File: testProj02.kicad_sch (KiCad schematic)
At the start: 25 parts, among them U1 24LC1025, U2 DS1337S_, U3 24LC1025, U4 ATMEGA328P-AU, Y1 32.768 KHZ, Y2 16 Mhz

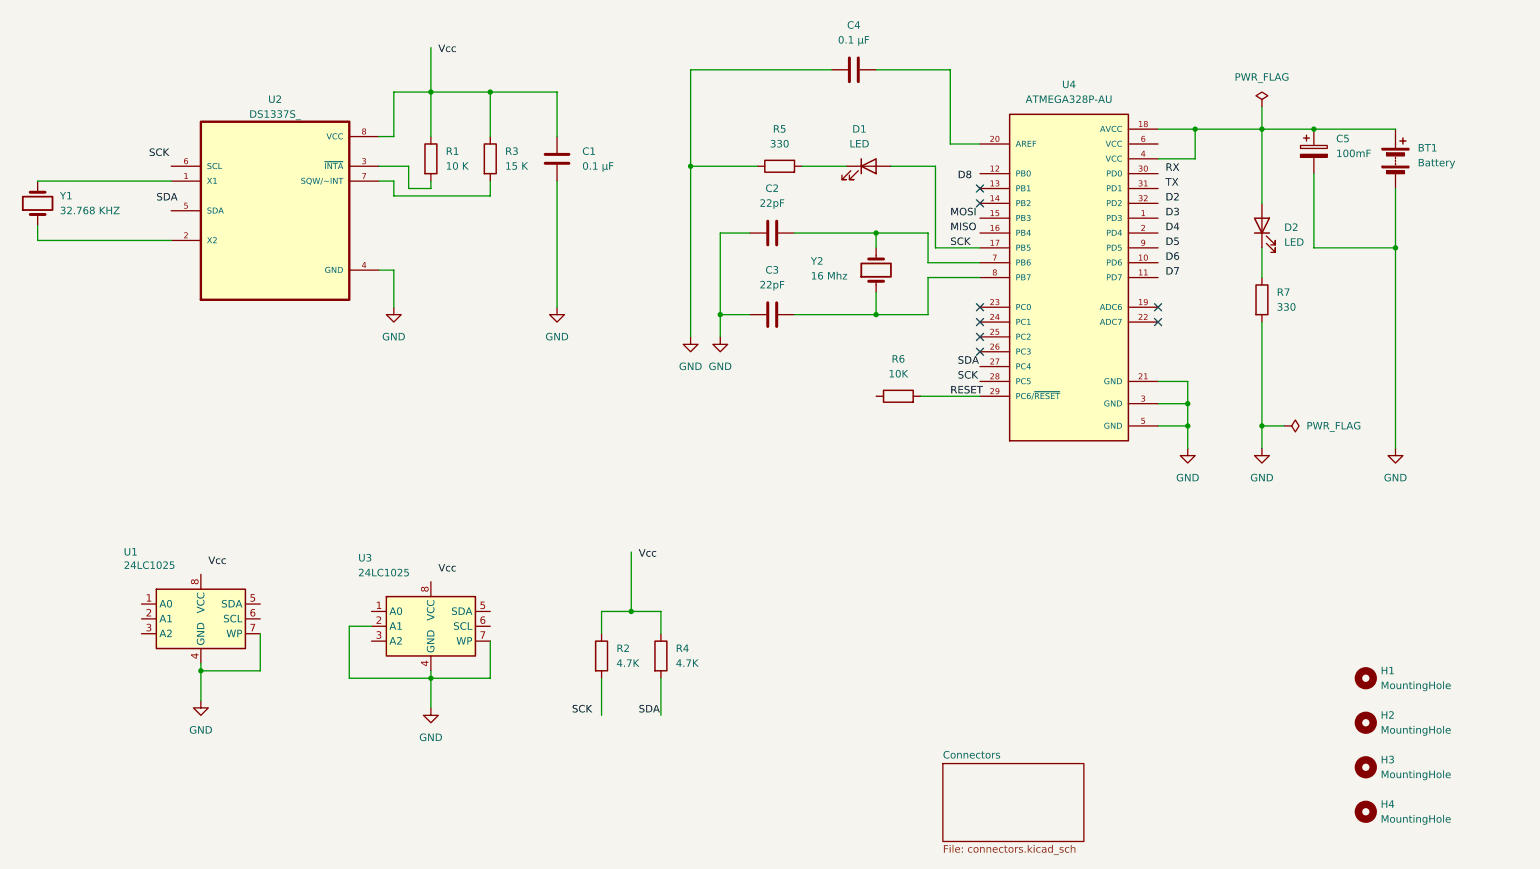
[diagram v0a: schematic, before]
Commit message: completed comments
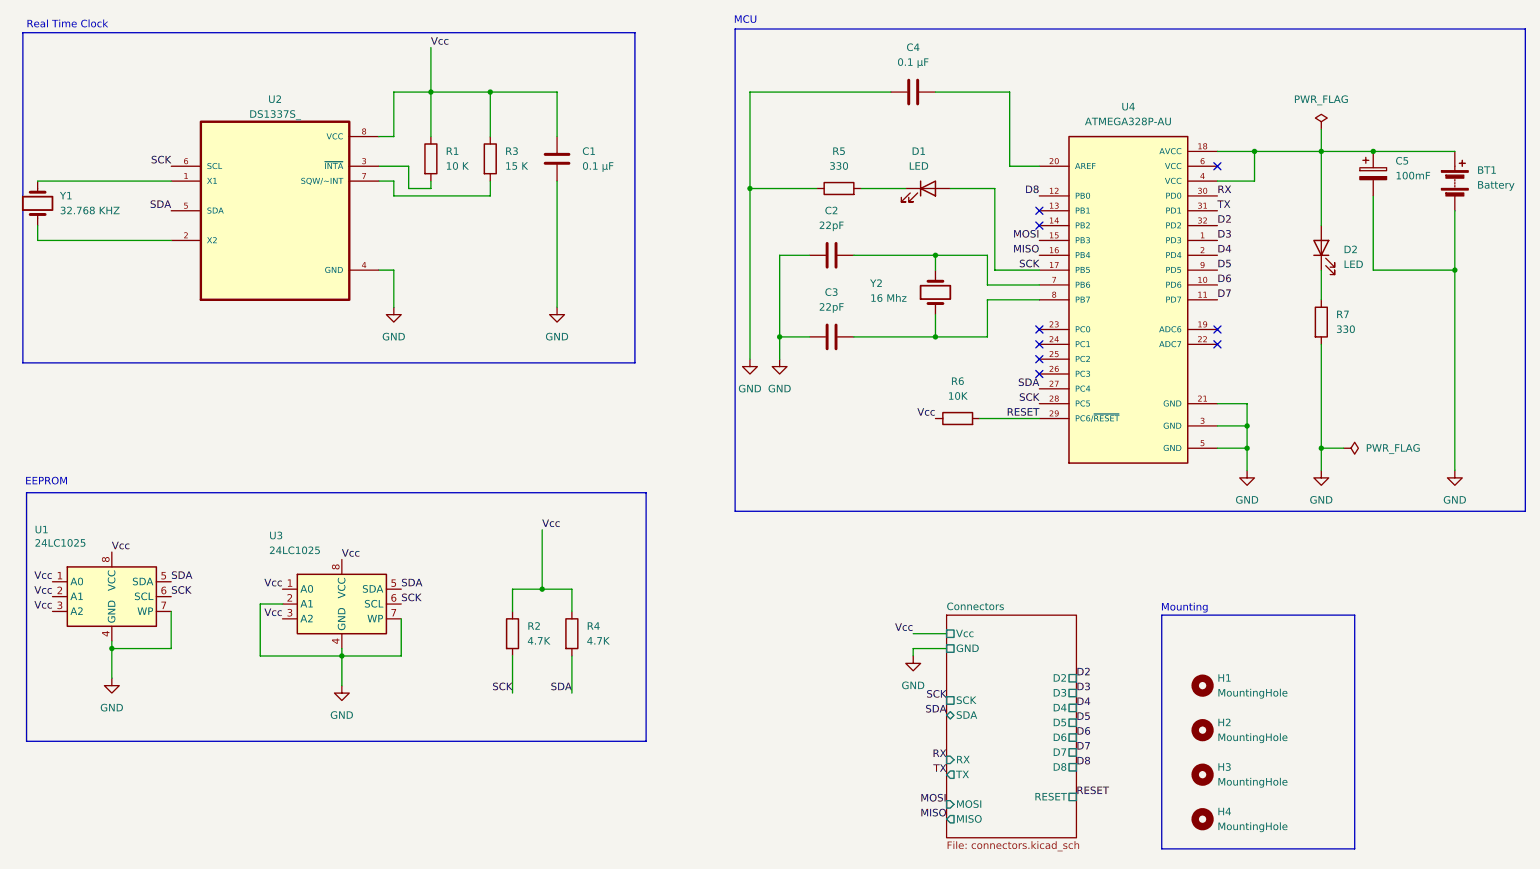
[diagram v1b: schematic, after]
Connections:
- net D2: now also U4.32 (PD2)
- net D3: now also U4.1 (PD3)
- net D4: now also U4.2 (PD4)
- net D5: now also U4.9 (PD5)
- net D6: now also U4.10 (PD6)
- net D7: now also U4.11 (PD7)
- net D8: now also U4.12 (PB0)
- net MISO: now also U4.16 (PB4)
- net MOSI: now also U4.15 (PB3)
- net RX: now also U4.30 (PD0)
- net SCK: now also R2.2, U1.6 (SCL), U2.6 (SCL), U3.6 (SCL), U4.28 (PC5)
- net SDA: now also R4.2, U1.5 (SDA), U2.5 (SDA), U3.5 (SDA), U4.27 (PC4)
- net TX: now also U4.31 (PD1)
- net Vcc: now also C1.1, R1.1, R2.1, R3.1, R4.1, R6.1, U1.1 (A0), U1.2 (A1), U1.3 (A2), U1.8 (VCC), U2.8 (VCC), U3.1 (A0), U3.3 (A2), U3.8 (VCC)
- no-connect marks 8 -> 9
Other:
- sheet Connectors ports: added D2, D3, D4, D5, D6, D7, D8, GND, MISO, MOSI, RESET, RX, SCK, SDA, TX, Vcc; removed none
- note added: "EEPROM"
- note added: "MCU"
- note added: "Mounting"
- note added: "Real Time Clock"
- moved on the sheet: BT1, C2, C3, C4, C5, D1, D2, H1, H2, H3, H4, R2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
